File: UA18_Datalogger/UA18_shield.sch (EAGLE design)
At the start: 5 parts, among them IC1 4067D, IC2 4067D, U2 ARDUINOR3-DIMENSION

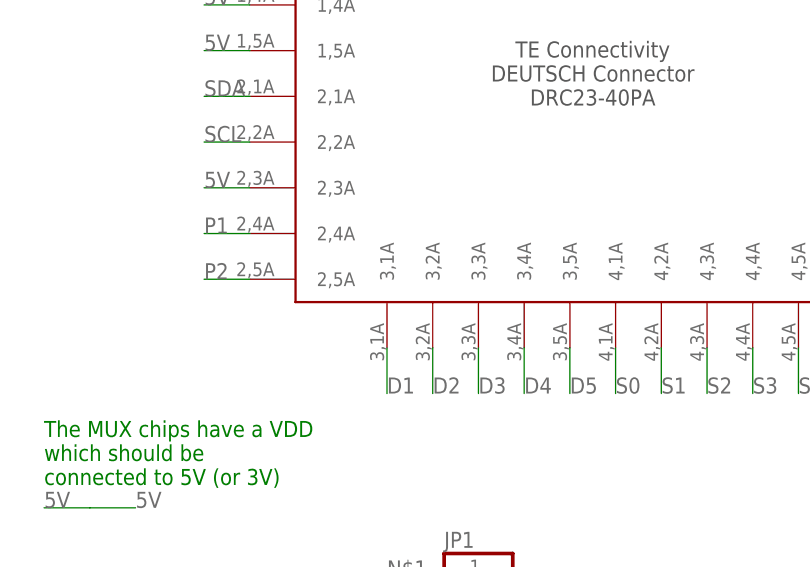
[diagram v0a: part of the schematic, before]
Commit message: finished datalogger
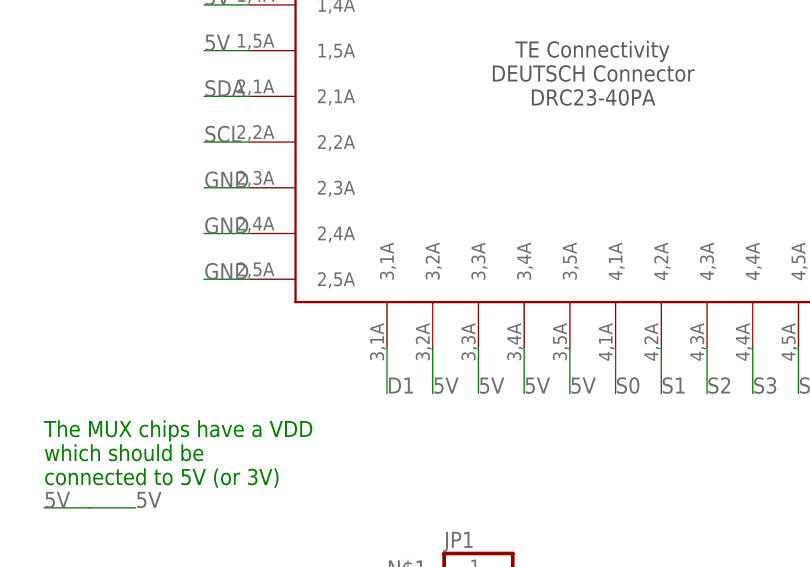
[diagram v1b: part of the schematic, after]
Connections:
- removed net D2: U$1.3,2A
- removed net D3: U$1.3,3A
- removed net D4: U$1.3,4A
- removed net D5: U$1.3,5A
- removed net P1: U$1.2,4A
- removed net P2: U$1.2,5A
- net 5V: now also U$1.3,2A, U$1.3,3A, U$1.3,4A, U$1.3,5A; no longer U$1.2,3A
- net GND: now also U$1.2,3A, U$1.2,4A, U$1.2,5A
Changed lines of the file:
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@@
 <?xml version="1.0" encoding="utf-8"?>
 <!DOCTYPE eagle SYSTEM "eagle.dtd">
-<eagle version="8.2.0">
+<eagle version="8.6.1">
 <drawing>
 <settings>
 <setting alwaysvectorfont="no"/>
+<setting keepoldvectorfont="yes"/>
 <setting verticaltext="up"/>
 </settings>
@@
 <label x="127" y="-106.68" size="1.778" layer="95"/>
 </segment>
+<segment>
+<pinref part="U$1" gate="G$1" pin="2,3A"/>
+<wire x1="111.76" y1="-48.26" x2="106.68" y2="-48.26" width="0.1524" layer="91"/>
+<label x="106.68" y="-48.26" size="1.778" layer="95"/>
+</segment>
+<segment>
+<pinref part="U$1" gate="G$1" pin="2,4A"/>
+<wire x1="111.76" y1="-53.34" x2="106.68" y2="-53.34" width="0.1524" layer="91"/>
+<label x="106.68" y="-53.34" size="1.778" layer="95"/>
+</segment>
+<segment>
+<pinref part="U$1" gate="G$1" pin="2,5A"/>
+<wire x1="111.76" y1="-58.42" x2="106.68" y2="-58.42" width="0.1524" layer="91"/>
+<label x="106.68" y="-58.42" size="1.778" layer="95"/>
+</segment>
 </net>
 <net name="SCL" class="0">
@@
 <wire x1="111.76" y1="-33.02" x2="106.68" y2="-33.02" width="0.1524" layer="91"/>
 <label x="106.68" y="-33.02" size="1.778" layer="95"/>
-</segment>
-<segment>
-<pinref part="U$1" gate="G$1" pin="2,3A"/>
-<wire x1="111.76" y1="-48.26" x2="106.68" y2="-48.26" width="0.1524" layer="91"/>
-<label x="106.68" y="-48.26" size="1.778" layer="95"/>
 </segment>
 <segment>
@@
 <wire x1="93.98" y1="-83.82" x2="88.9" y2="-83.82" width="0.1524" layer="91"/>
 </segment>
+<segment>
+<pinref part="U$1" gate="G$1" pin="3,2A"/>
+<wire x1="132.08" y1="-66.04" x2="132.08" y2="-71.12" width="0.1524" layer="91"/>
+<label x="132.08" y="-71.12" size="1.778" layer="95"/>
+</segment>
+<segment>
+<pinref part="U$1" gate="G$1" pin="3,3A"/>
+<wire x1="137.16" y1="-66.04" x2="137.16" y2="-71.12" width="0.1524" layer="91"/>
+<label x="137.16" y="-71.12" size="1.778" layer="95"/>
+</segment>
+<segment>
+<pinref part="U$1" gate="G$1" pin="3,4A"/>
+<wire x1="142.24" y1="-66.04" x2="142.24" y2="-71.12" width="0.1524" layer="91"/>
+<label x="142.24" y="-71.12" size="1.778" layer="95"/>
+</segment>
+<segment>
+<pinref part="U$1" gate="G$1" pin="3,5A"/>
+<wire x1="147.32" y1="-66.04" x2="147.32" y2="-71.12" width="0.1524" layer="91"/>
+<label x="147.32" y="-71.12" size="1.778" layer="95"/>
+</segment>
 </net>
 <net name="3V" class="0">
@@
 </segment>
 </net>
-<net name="P1" class="0">
-<segment>
-<pinref part="U$1" gate="G$1" pin="2,4A"/>
-<wire x1="111.76" y1="-53.34" x2="106.68" y2="-53.34" width="0.1524" layer="91"/>
-<label x="106.68" y="-53.34" size="1.778" layer="95"/>
-</segment>
-</net>
-<net name="P2" class="0">
-<segment>
-<pinref part="U$1" gate="G$1" pin="2,5A"/>
-<wire x1="111.76" y1="-58.42" x2="106.68" y2="-58.42" width="0.1524" layer="91"/>
-<label x="106.68" y="-58.42" size="1.778" layer="95"/>
-</segment>
-</net>
 <net name="D1" class="0">
 <segment>
@@
 <wire x1="71.12" y1="-109.22" x2="76.2" y2="-109.22" width="0.1524" layer="91"/>
 <label x="73.66" y="-109.22" size="1.778" layer="95"/>
-</segment>
-</net>
-<net name="D2" class="0">
-<segment>
-<pinref part="U$1" gate="G$1" pin="3,2A"/>
-<wire x1="132.08" y1="-66.04" x2="132.08" y2="-71.12" width="0.1524" layer="91"/>
-<label x="132.08" y="-71.12" size="1.778" layer="95"/>
-</segment>
-</net>
-<net name="D3" class="0">
-<segment>
-<pinref part="U$1" gate="G$1" pin="3,3A"/>
-<wire x1="137.16" y1="-66.04" x2="137.16" y2="-71.12" width="0.1524" layer="91"/>
-<label x="137.16" y="-71.12" size="1.778" layer="95"/>
-</segment>
-</net>
-<net name="D4" class="0">
-<segment>
-<pinref part="U$1" gate="G$1" pin="3,4A"/>
-<wire x1="142.24" y1="-66.04" x2="142.24" y2="-71.12" width="0.1524" layer="91"/>
-<label x="142.24" y="-71.12" size="1.778" layer="95"/>
-</segment>
-</net>
-<net name="D5" class="0">
-<segment>
-<pinref part="U$1" gate="G$1" pin="3,5A"/>
-<wire x1="147.32" y1="-66.04" x2="147.32" y2="-71.12" width="0.1524" layer="91"/>
-<label x="147.32" y="-71.12" size="1.778" layer="95"/>
 </segment>
 </net>
@@
 </note>
 <note version="8.2" severity="warning">
-Since Version 8.2, Eagle supports online libraries. The ids
+Since Version 8.2, EAGLE supports online libraries. The ids
 of those online libraries will not be understood (or retained)
 with this version.
